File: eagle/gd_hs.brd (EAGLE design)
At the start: 108 x 108 mm, 60 parts, among them K1 G5V-2, X4 BU-SMA-V

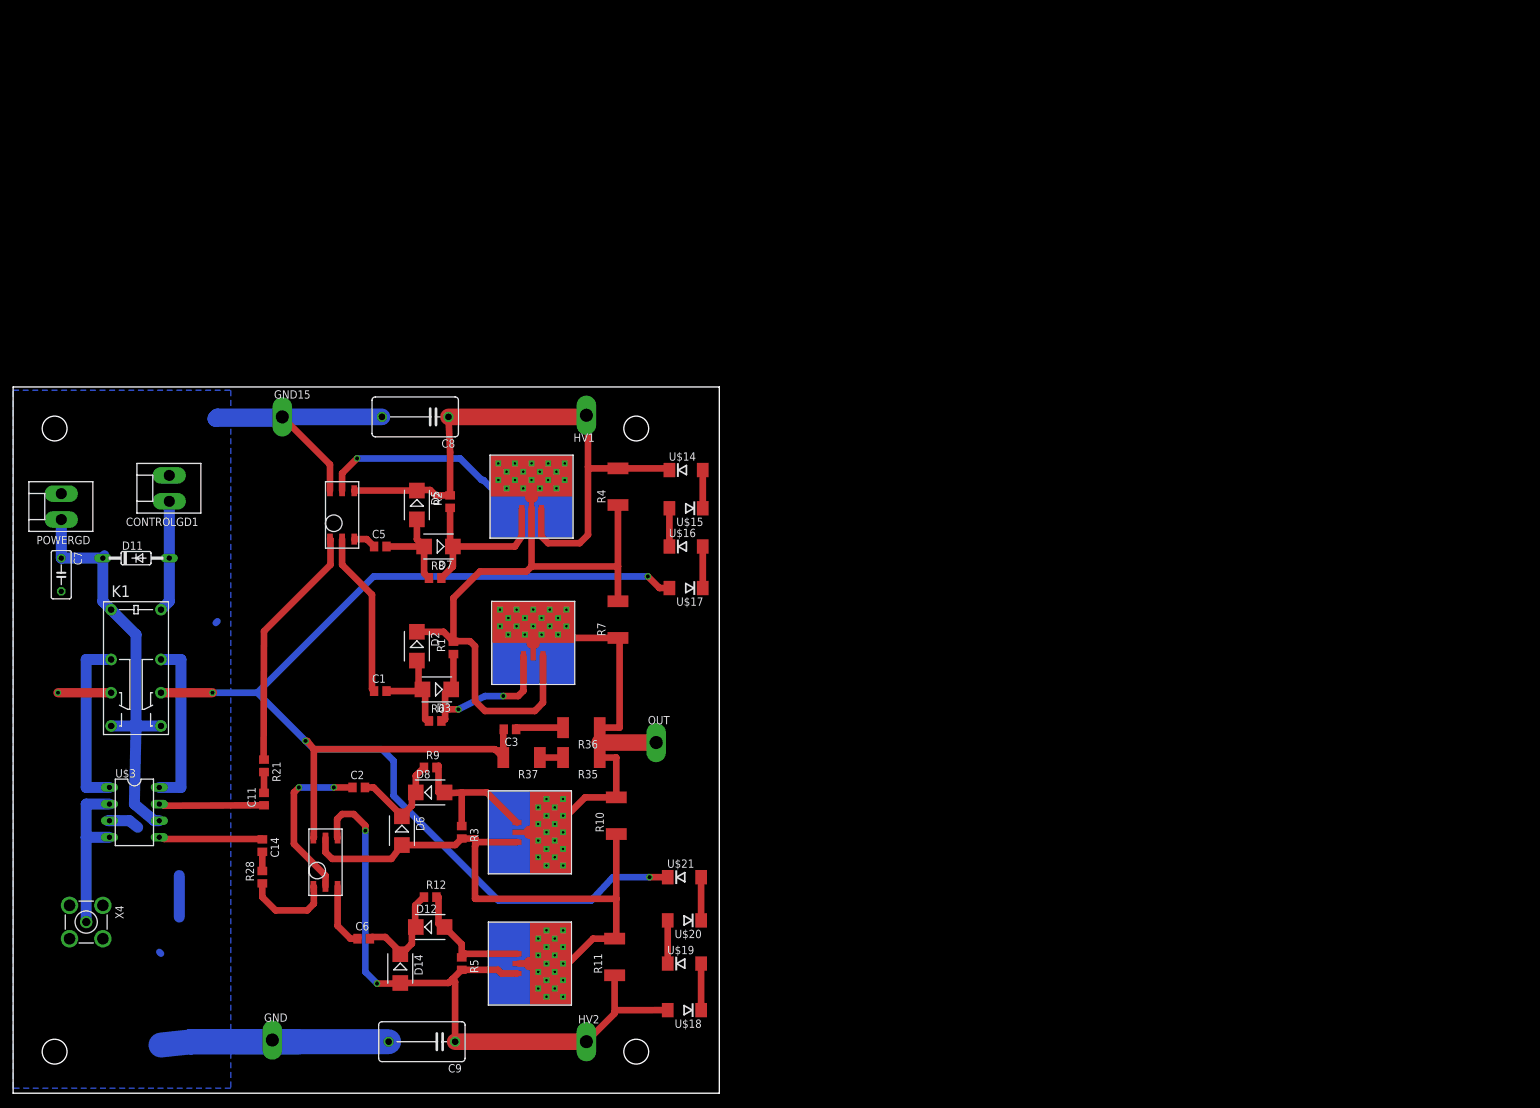
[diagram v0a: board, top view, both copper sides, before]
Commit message: code, simulations, heat sink layout
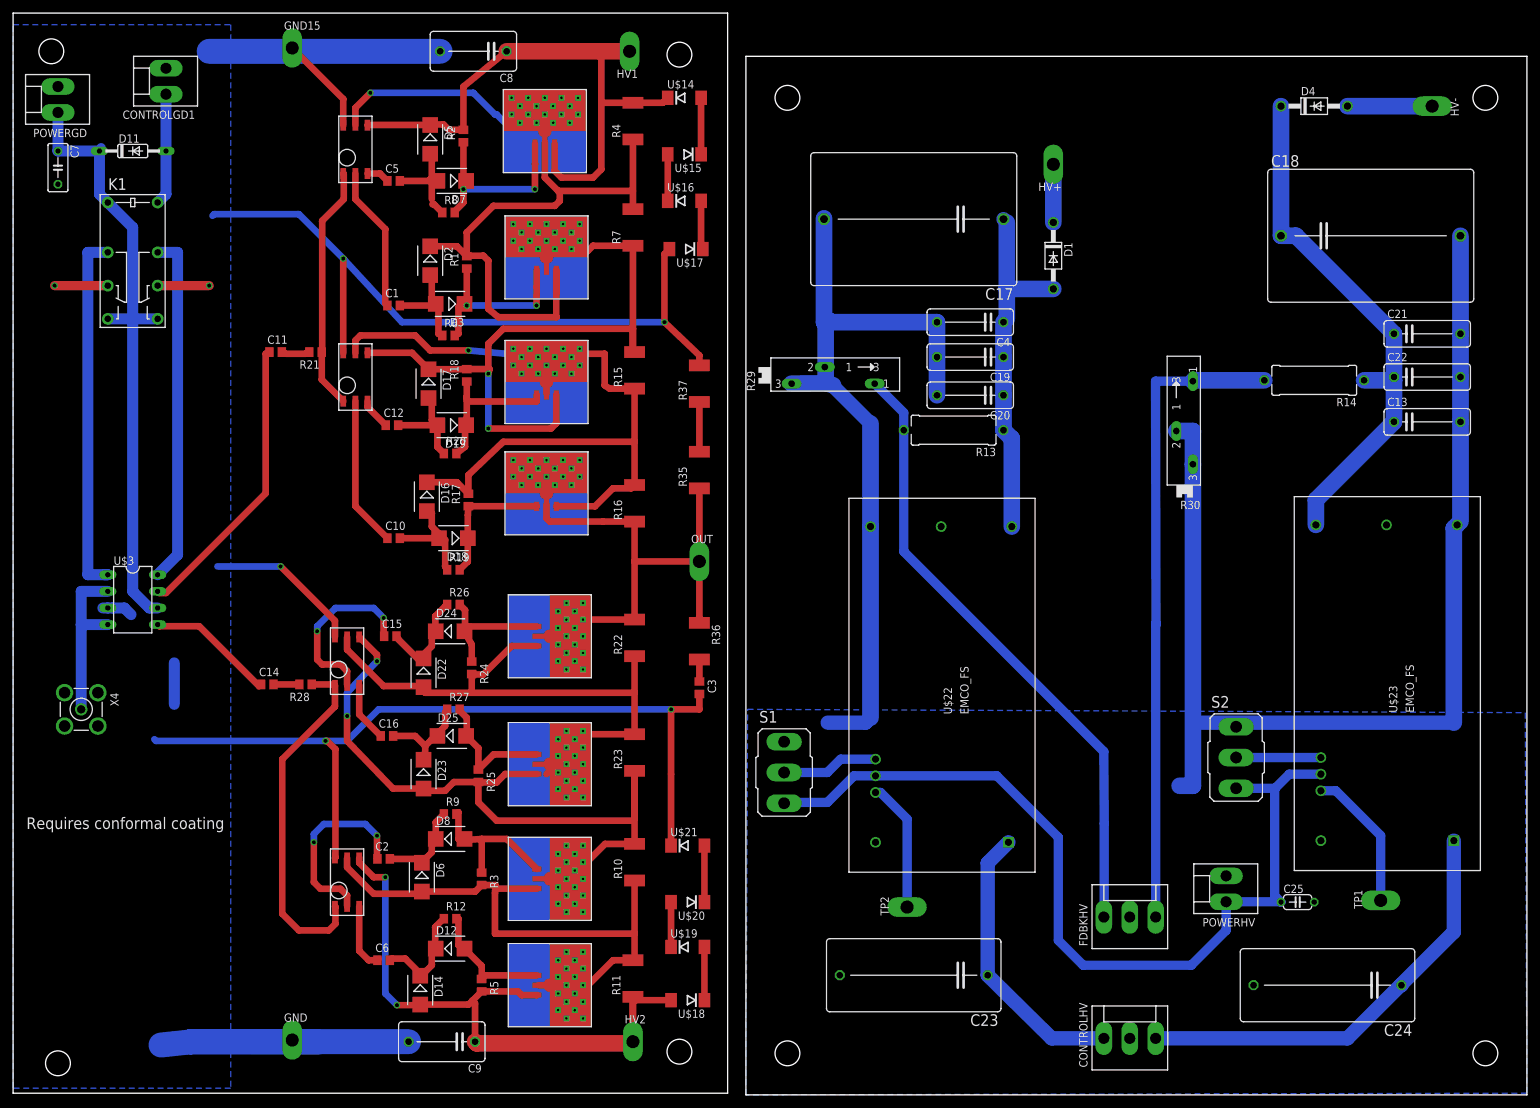
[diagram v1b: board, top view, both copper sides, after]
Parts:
- added C10, C12, C15, C16: 1u, resistor:C0805
- added C13, C4: .01u, rcl:C102-043X133
- added C17, C18: 1u, rcl:C275-205X316
- added C19, C21: 1n, rcl:C102-043X133
- added C20, C22: 10p, rcl:C102-043X133
- added C23, C24: .1u, rcl:C225-113X268
- added C25: 10n, rcl:C050-024X044
- added CONTROLHV, FDBKHV: (no value), con-molex:KK-156-3
- added D1, D4: 1N4004, diode:DO41-10
- added D16, D17, D22, D23: 1SMB5918BT3G, diode:SMB
- added D18, D19, D24, D25: (no value), diode:SMB
- added HV+, HV-: TPPAD1-20Y, testpad:P1-20Y
- added POWERHV: (no value), con-molex:KK-156-2
- added R13, R14: 2M, resistor:P0613/15
- added R15, R16, R22, R23: 10M, rcl:R2512
- added R17, R18, R24, R25: 100k, rcl:R0805
- added R19, R20, R26, R27: 10, rcl:R0805
- added R29, R30: (no value), pot:SP19L
- added S1, S2: (no value), switch:M9040P
- added TP1, TP2: PTR1PAD1-20Y, testpad:P1-20Y
- added U$10, U$9: VP2450HS, transistor-fet:SO89_HS
- added U$11, U$12: VN2450HS, transistor-fet:SO89_HS
- added U$13, U$8: DA-2320SMD6, trafo:SMD6
- added U$22, U$23: EMCO-FS10, dc-dc-converter:EMCO-FS
- moved C11 68.3 mm to (40.1, 113.3), turned to 0 degrees
- moved R21 63.7 mm to (46.2, 113.3), turned to 180 degrees
- moved R37 63.3 mm to (104.9, 108.5), turned to 90 degrees
- moved C7 62.2 mm to (6.86, 141.5)
- moved CONTROLGD1 62.2 mm to (23.4, 154.7)
- moved D11 62.2 mm to (18.3, 144.0)
- moved K1 62.2 mm to (18.3, 127.3)
- moved POWERGD 62.2 mm to (6.86, 151.9)
- moved R7 60.0 mm to (94.7, 132.3)
- moved D2 59.0 mm to (63.8, 127.3)
- moved D3 59.0 mm to (66.8, 120.7)
- moved C1 59.0 mm to (58.2, 120.4)
- moved R1 59.0 mm to (69.3, 127.0)
- moved R6 59.0 mm to (66.5, 115.8)
- moved U$5 59.0 mm to (81.5, 127.8)
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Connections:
- new net +5V: C25.1, POWERHV.1, S1.3, S2.3, U$22.+5, U$23.+5
- new net GND1: C13.2, C17.2, C18.2, C19.2, C20.2, C21.2, C22.2, C23.2, C24.2, C25.2, C4.2, CONTROLHV.2, FDBKHV.2, POWERHV.2, R29.E, R29.S, R30.E, R30.S, S1.1, S2.1, U$22.-IN, U$22.-OUT, U$23.+OUT, U$23.-IN
- new net N$13: C17.1, C19.1, C20.1, C4.1, D1.A, R13.1, U$22.+OUT
- new net N$17: C13.1, C18.1, C21.1, C22.1, D4.C, R14.1, U$23.-OUT
- new net N$18: FDBKHV.1, R13.2, R29.A
- new net N$19: FDBKHV.3, R14.2, R30.A
- new net N$24: D1.C, HV+.TP
- new net N$26: OUT.TP, R16.1, R22.2, R35.1, R36.1, U$10.C, U$10.C@1, U$11.C, U$11.C@1
- new net N$28: C10.1, U$8.P$2
- new net N$29: C12.1, U$8.P$3
- new net N$3: D16.C, R15.1, R16.2, R17.2, U$10.E, U$8.P$5, U$9.C, U$9.C@1
- new net N$30: C12.2, D17.A, D19.A, R20.1
- new net N$32: D4.A, HV-.TP
- new net N$33: C23.1, CONTROLHV.1, U$22.+IN
- new net N$34: D18.C, R17.1, R19.2, U$10.B
- new net N$35: C10.2, D16.A, D18.A, R19.1
- new net N$36: D19.C, R18.1, R20.2, U$9.B
- new net N$40: C15.1, U$13.P$2
- new net N$41: C16.1, U$13.P$3
- new net N$42: C15.2, D22.C, D24.C, R26.1
- new net N$43: C16.2, D23.C, D25.C, R27.1
- new net N$46: D22.A, R22.1, R23.2, R24.2, U$11.E, U$12.C, U$12.C@1, U$13.P$5
- new net N$47: D25.A, R25.1, R27.2, U$12.B
- new net N$50: D24.A, R24.1, R26.2, U$11.B
- new net N$51: C24.1, CONTROLHV.3, U$23.+IN
- new net N$57: D17.C, R15.2, R18.2, R7.1, U$5.C, U$5.C@1, U$8.P$4, U$9.E
- new net N$58: TP1.TP, U$23.ALARM
- new net N$59: TP2.TP, U$22.ALARM
- new net N$60: S1.2, U$22.DISABLE
- new net N$61: S2.2, U$23.DISABLE
- net GND: now also U$13.P$6, U$8.P$6
- net N$20: now also D23.A, R23.1, R25.2, U$12.E, U$13.P$4; no longer OUT.TP, R35.1, R36.1, R7.1, U$5.C, U$5.C@1
- net N$37: now also U$8.P$1
- net N$48: now also U$13.P$1
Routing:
- net GND1: track 0.00 -> 340.6 mm
- net +5V: track 0.00 -> 137.3 mm
- net N$3: track 0.00 -> 122.0 mm, vias 0 -> 1
- net N$57: track 0.00 -> 104.7 mm, vias 0 -> 2
- net N$19: track 0.00 -> 98.9 mm
- net N$18: track 0.00 -> 96.1 mm
- net N$46: track 0.00 -> 89.4 mm
- net N$17: track 0.00 -> 82.0 mm
- net N$26: track 0.00 -> 75.4 mm
- net N$51: track 0.00 -> 66.3 mm
- net GND: track 339.1 -> 398.8 mm, vias 5 -> 7
- net N$13: track 0.00 -> 55.0 mm
- net N$20: track 70.1 -> 116.7 mm, vias 0 -> 2
- net N$33: track 0.00 -> 43.4 mm
- net N$48: track 13.9 -> 54.1 mm
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- added copper zone on layer 16, net GND1
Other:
- board size 108 x 108 mm -> 231.4 x 165.4 mm
- board text added: "Requires conformal coating"
